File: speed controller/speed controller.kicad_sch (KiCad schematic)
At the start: 1 part

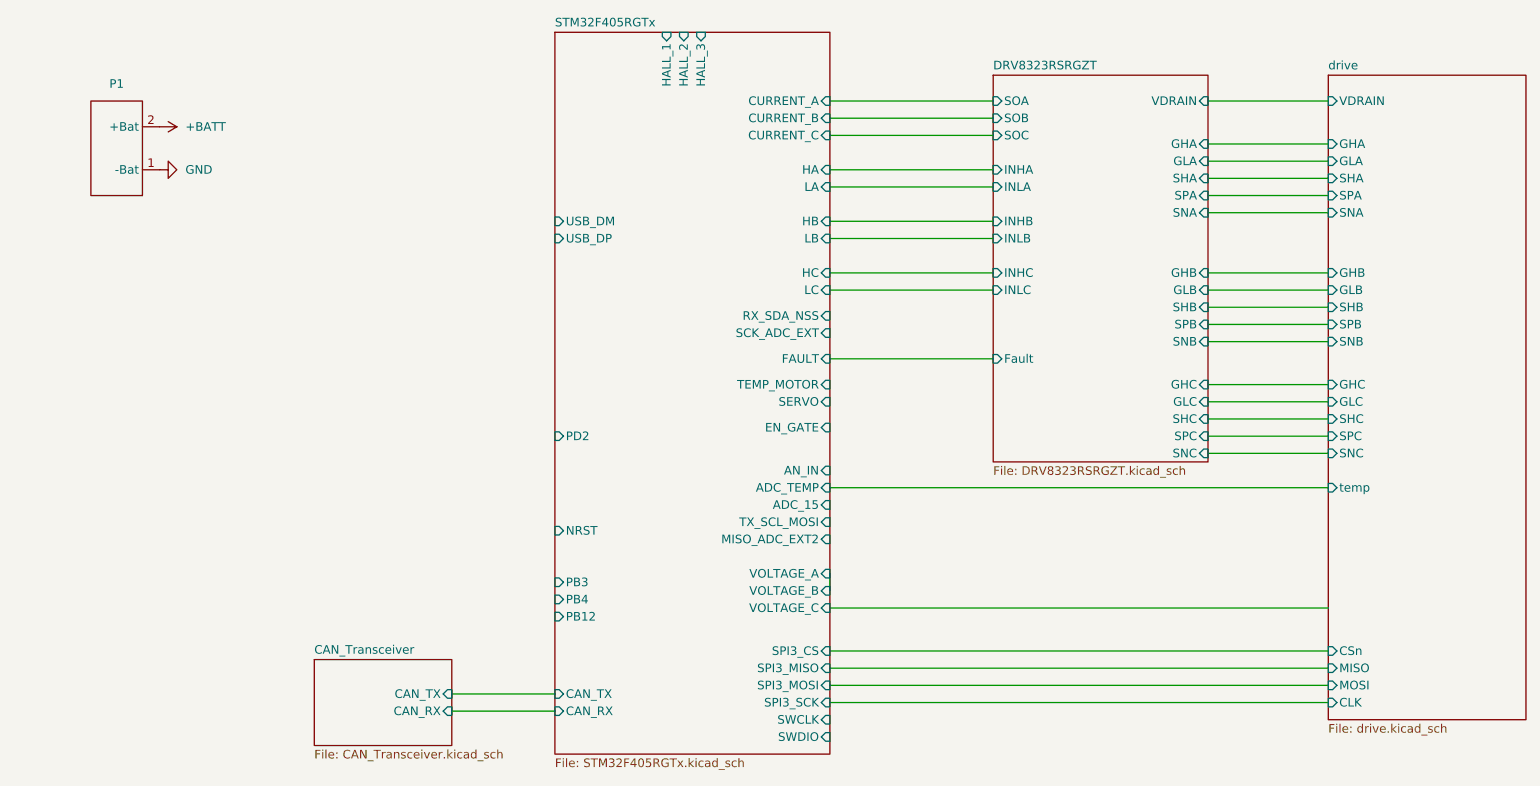
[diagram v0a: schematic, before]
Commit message: inital board layout
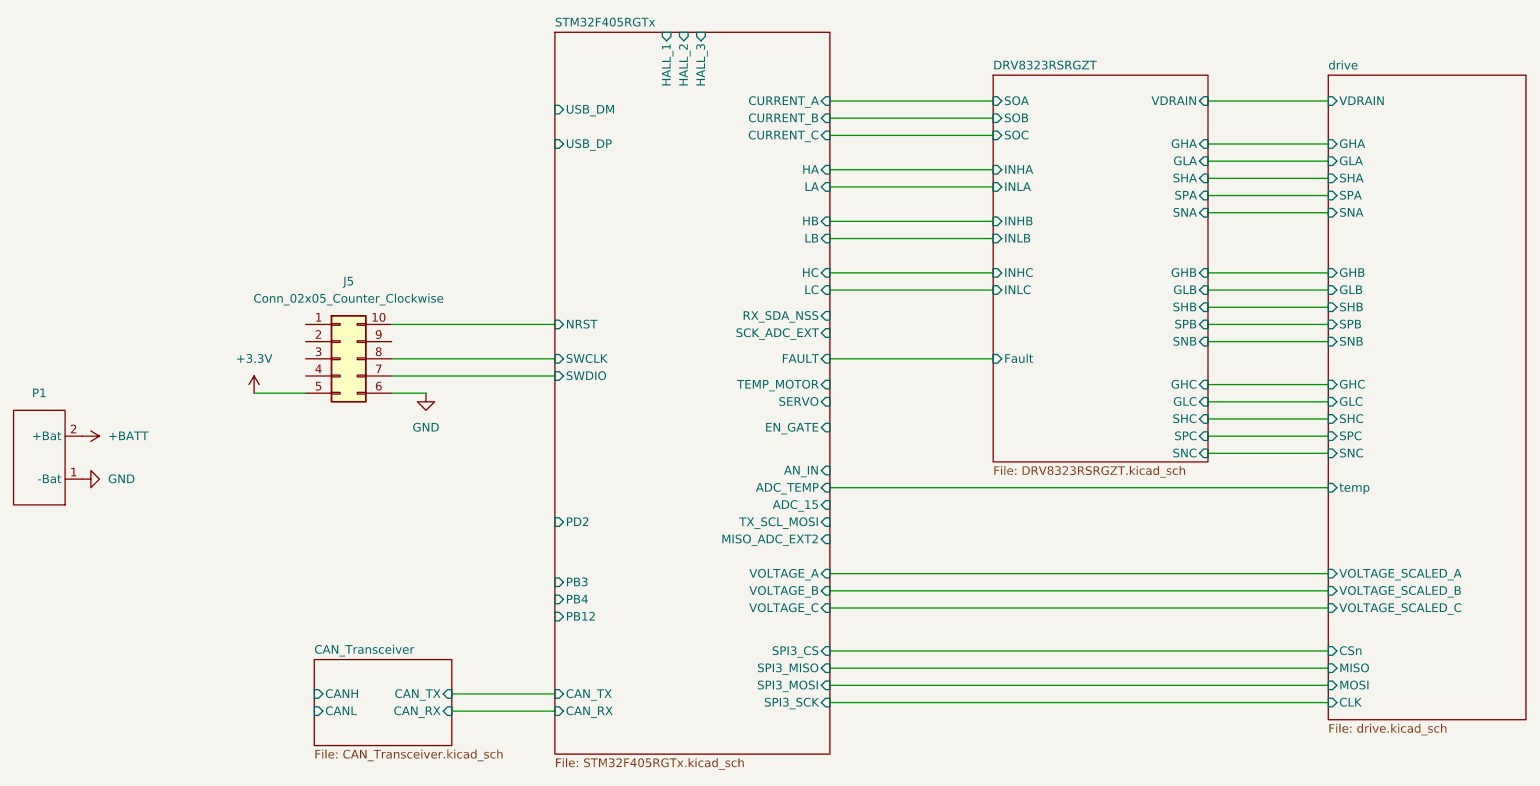
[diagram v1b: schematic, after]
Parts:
- added J5: Conn_02x05_Counter_Clockwise, Connector_PinHeader_1.27mm:PinHeader_2x05_P1.27mm_Vertical, symbol Connector_Generic:Conn_02x05_Counter_Clockwise
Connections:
- net GND: now also J5.6 (Pin_6)
- net STM32F405RGTx/NRST: now also J5.10 (Pin_10)
- net STM32F405RGTx/SWCLK: now also J5.8 (Pin_8)
- net STM32F405RGTx/SWDIO: now also J5.7 (Pin_7)
- new net +3.3V: J5.5 (Pin_5)
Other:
- sheet CAN_Transceiver ports: added CANH, CANL; removed none
- sheet drive ports: added VOLTAGE_SCALED_A, VOLTAGE_SCALED_B, VOLTAGE_SCALED_C; removed none
- moved on the sheet: P1
